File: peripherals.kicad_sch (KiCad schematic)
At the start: 29 parts, among them J4 OLED I2C, J8 Conn_01x06, U10 ESP32-S3-MINI-1-N8, U5 M24M02-DRMN6TP

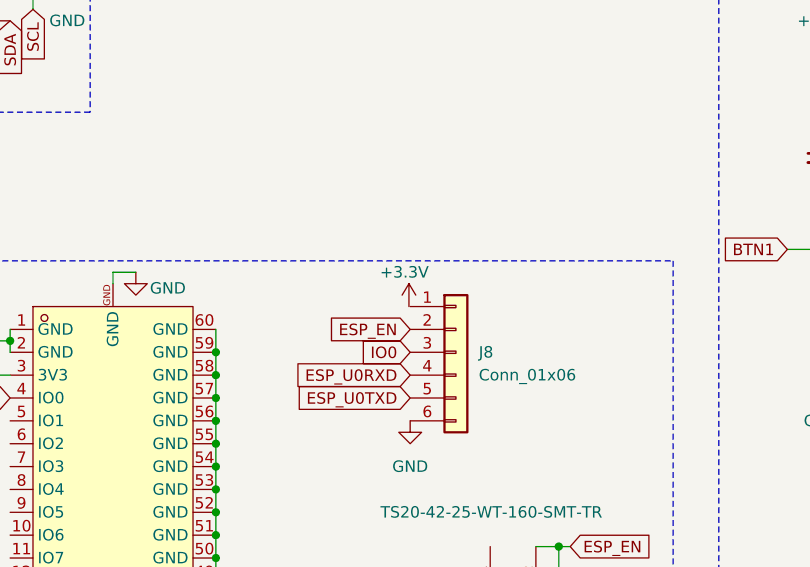
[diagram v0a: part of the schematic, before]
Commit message: slightly change schematic, making sure everything is ok, preparing for finalization
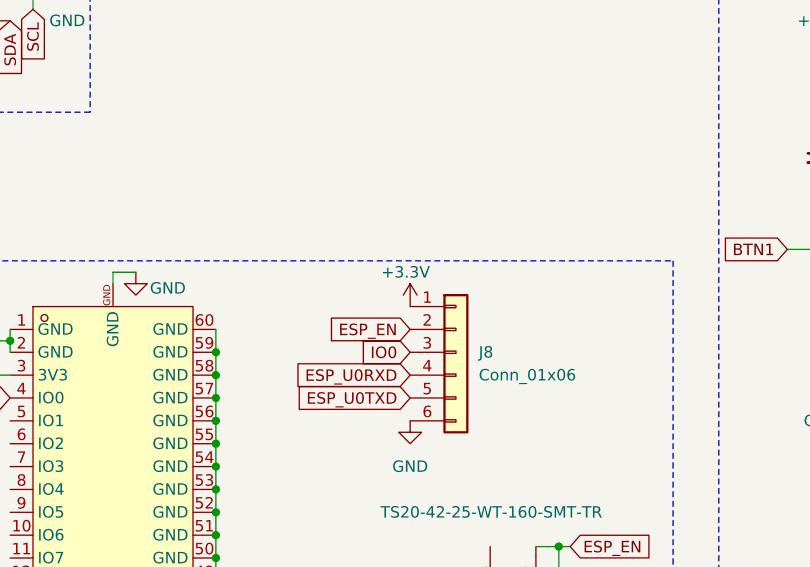
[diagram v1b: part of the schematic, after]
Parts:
- J4: footprint Connector_PinSocket_2.54mm:PinSocket_2x04_P2.54mm_Horizontal -> Connector_PinSocket_2.54mm:PinSocket_2x04_P2.54mm_Vertical
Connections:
- net +3.3V: now also J8.1 (Pin_1)
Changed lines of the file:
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@@
 			)
 		)
-		(property "Footprint" "Connector_PinSocket_2.54mm:PinSocket_2x04_P2.54mm_Horizontal"
+		(property "Footprint" "Connector_PinSocket_2.54mm:PinSocket_2x04_P2.54mm_Vertical"
 			(at 58.42 24.13 0)
 			(hide yes)
@@
 	(symbol
 		(lib_id "power:+3.3V")
-		(at 109.0833 99.06 0)
+		(at 109.22 99.06 0)
 		(unit 1)
 		(body_style 1)
@@
 		(dnp no)
 		(property "Reference" "#PWR0140"
-			(at 109.0833 102.87 0)
+			(at 109.22 102.87 0)
 			(hide yes)
 			(show_name no)
@@
 		)
 		(property "Value" "+3.3V"
-			(at 108.5753 95.25 0)
+			(at 108.712 95.25 0)
 			(show_name no)
 			(do_not_autoplace no)
@@
 		)
 		(property "Footprint" ""
-			(at 109.0833 99.06 0)
-			(hide yes)
-			(show_name no)
-			(do_not_autoplace no)
-			(effects
-				(font
-					(size 1.27 1.27)
-				)
-			)
-		)
-		(property "Datasheet" ""
-			(at 109.0833 99.06 0)
+			(at 109.22 99.06 0)
+			(hide yes)
+			(show_name no)
+			(do_not_autoplace no)
+			(effects
+				(font
+					(size 1.27 1.27)
+				)
+			)
+		)
+		(property "Datasheet" ""
+			(at 109.22 99.06 0)
 			(hide yes)
 			(show_name no)
@@
 		)
 		(property "Description" "Power symbol creates a global label with name \"+3.3V\""
-			(at 109.0833 99.06 0)
-			(hide yes)
-			(show_name no)
+			(at 109.22 99.06 0)
+			(hide yes)
+			(show_name no)
